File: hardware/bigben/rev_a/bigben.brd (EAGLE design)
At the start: 26.9 x 13 mm, 13 parts, among them J3 IMPULSE_GECKO_HEADER, U1 RV-3049-C3, U2 FM25LBTDFN-8

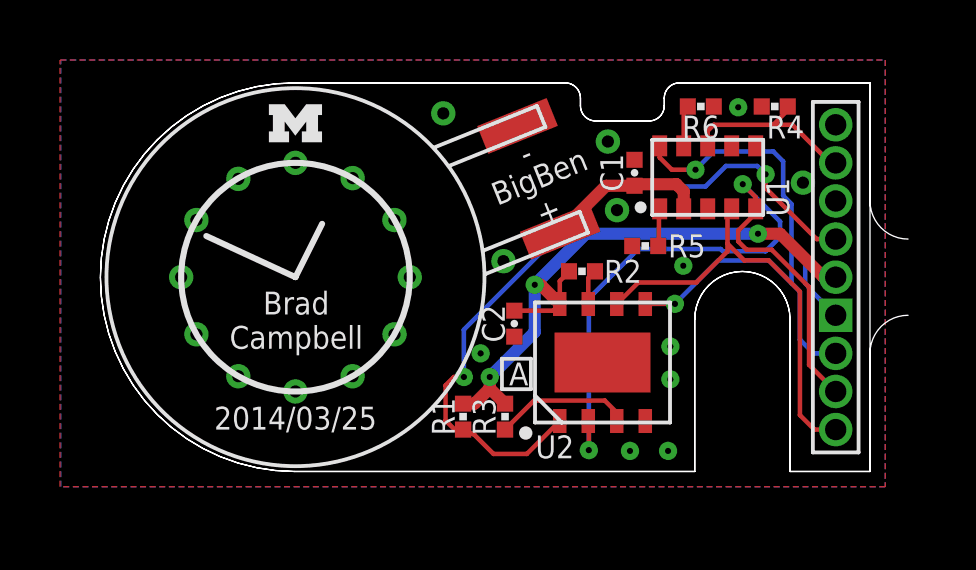
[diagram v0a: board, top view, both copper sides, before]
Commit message: shipped bigben
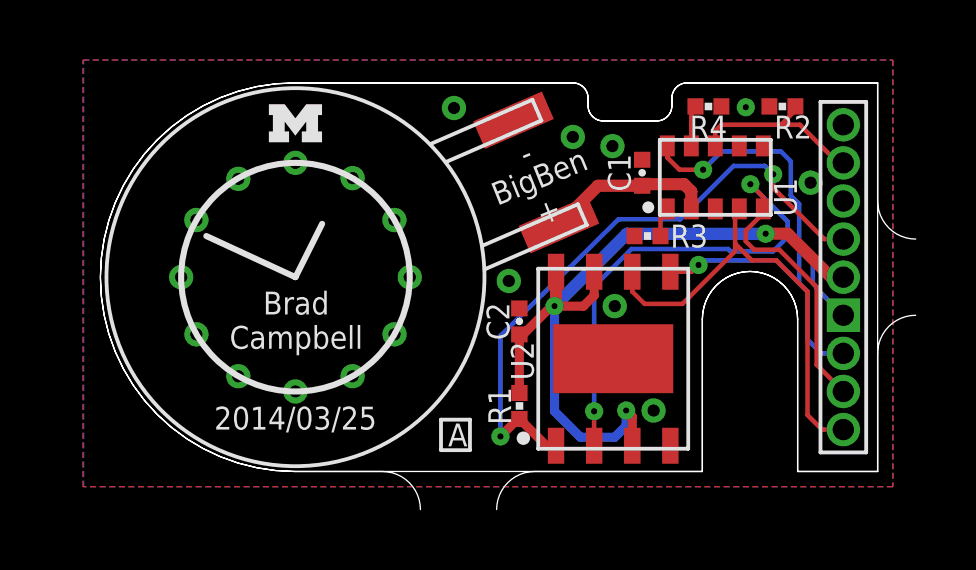
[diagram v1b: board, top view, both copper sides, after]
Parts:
- removed R5, R6: 10k, passives:0402_RES
- R3, R4: value 4.7k -> 10k
- U2: value FM25LBTDFN-8 -> FM25V20-DG; device chips:TDFN-8 -> chips:TDFN-8/6MM
- moved R2 8.65 mm to (22.7, 12.2), turned to 0 degrees
- moved R3 7.67 mm to (18.2, 7.85), turned to 0 degrees
- moved R4 2.21 mm to (20.3, 12.2), turned to 180 degrees
- moved R1 1.91 mm to (14.0, 2.18)
- moved U2 0.38 mm to (17.1, 3.76)
- moved C1 0.25 mm to (18.1, 9.96)
- moved J3 0.25 mm to (24.8, 6.48)
- moved U1 0.25 mm to (20.5, 9.80)
- moved C2 0.18 mm to (14.0, 5.00), turned to 90 degrees
- turned BT1 to 23.5 degrees
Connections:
- removed net !FRAM_HOLD: R2.1, U2.7
- removed net !FRAM_WP: R3.1, U2.3
- net GND: now also R2.1, R3.1; no longer R5.1, R6.1
- net N$6: now also R4.2; no longer R6.2
- net N$7: now also R3.2; no longer R5.2
- net RTC_CS: now also R2.2; no longer R4.2
- net VCC: now also U2.3, U2.7; no longer R2.2, R3.2
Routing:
- net VCC: track 21.2 -> 26.3 mm
- net !FRAM_WP: track 4.57 -> 0.00 mm
- net !FRAM_CS: track 24.1 -> 20.9 mm
- net !FRAM_HOLD: track 1.18 -> 0.00 mm
- net MOSI0: track 18.4 -> 17.4 mm
- net MISO0: track 24.8 -> 23.9 mm
- net SCLK0: track 14.5 -> 15.0 mm
- net GND: vias 24 -> 20
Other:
- board size 26.9 x 13 mm -> 27.2 x 14.2 mm
